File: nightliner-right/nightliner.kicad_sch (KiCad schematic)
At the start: 90 parts, among them J1 TYPE-C-31-M-12, J2 Battery, J3 Serial, J4 Battery, P1 ISP_Prog, SW1 pinky_top, SW10 inner_home, SW11 pinky_bottom, SW12 ring_bottom, SW13 middle_bottom, SW14 index_bottom, SW15 inner_bottom, SW16 outer_top, SW17 outer_home, SW18 near_thumb, SW19 home_thumb, SW2 ring_top, SW20 far_thumb, SW21 ON_OFF, SW22 RESET, SW3 middle_top, SW4 index_top, SW5 inner_top, SW6 pinky_home, SW7 ring_home, SW8 middle_home, SW9 index_home, U1 holyiot-18010, U2 TVS2200DRV, U3 USBLC6-2SC6, U4 BQ24075RGT, U5 XC6220B331MR

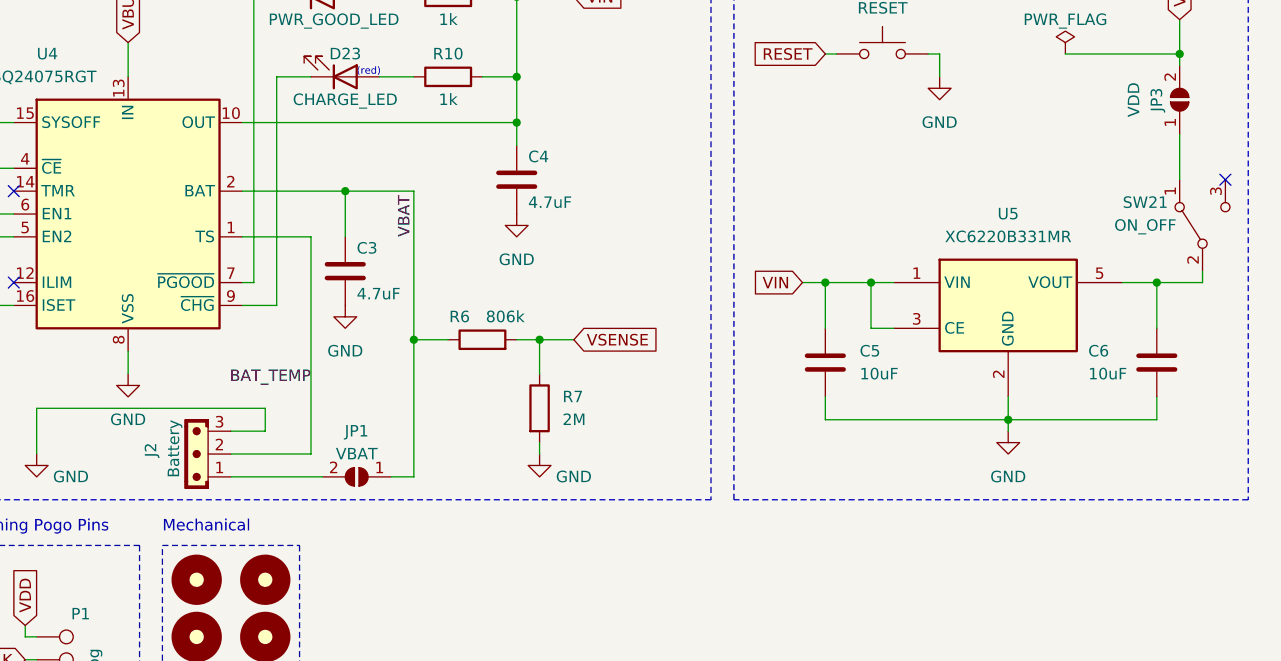
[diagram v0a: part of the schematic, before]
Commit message: fix: final version, create production gerbers
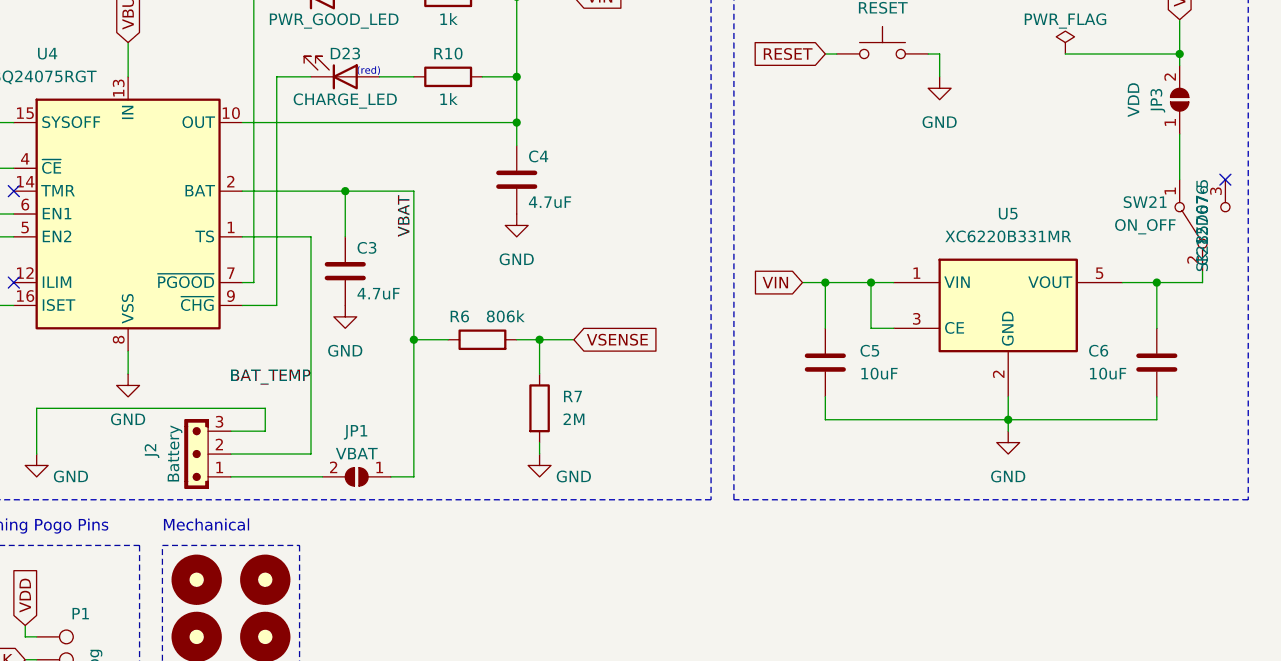
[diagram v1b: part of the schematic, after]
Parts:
- C1: LCSCNumber (none) -> C94121; PartNumber (none) -> CC0805KRX7R9BB102
- C2: LCSCNumber (none) -> C91186; PartNumber (none) -> CC0805KKX7R8BB105
- C3, C4: LCSCNumber (none) -> C354262; PartNumber (none) -> CC0805KKX7R8BB475
- C5, C6, C7: LCSCNumber (none) -> C89831; PartNumber (none) -> CC0805KKX5R8BB106
- D1, D10, D11, D12, D13, D14, D15, D16, D17, D18, D19, D2, D20, D3, D4, D5, D6, D7, D8, D9: value D_Small -> 1N4148WS; LCSCNumber (none) -> C5345963; PartNumber (none) -> 1N4148WS
- D25: LCSCNumber (none) -> C727115; PartNumber (none) -> 1N5819W
- H1: footprint miro_keyboard:StandOff_6mm_M3 -> nightliner:StandOff_6mm_M3
- H2, H3, H4, H5, H6, H7: value MountingHole_M3 -> Standoff_6mm_M3; footprint miro_keyboard:StandOff_6mm_M3 -> nightliner:StandOff_6mm_M3
- J1: symbol Connector:USB_C_Receptacle_USB2.0 -> nightliner:USB_C_Receptacle_USB2.0
- J2: LCSCNumber (none) -> C163036; PartNumber (none) -> S3B-XH-A-1(LF)(SN)
- J3: footprint miro_keyboard:MagConn_6pin_right -> nightliner:MagConn_6pin_right
- P1: footprint miro_keyboard:ISP_Programming_Pads -> nightliner:ISP_Programming_Pads
- R1, R2: LCSCNumber (none) -> C144553; PartNumber (none) -> AC0805FR-075K1L
- R10, R11, R8, R9: LCSCNumber (none) -> C95781; PartNumber (none) -> RC0805FR-071KL
- R3: LCSCNumber (none) -> C107700; PartNumber (none) -> RC0805FR-071ML
- R4: LCSCNumber (none) -> C140868; PartNumber (none) -> AC0805FR-0710KL
- R6: LCSCNumber (none) -> C273852; PartNumber (none) -> RC0805FR-07806KL
- R7: LCSCNumber (none) -> C114532; PartNumber (none) -> RC0805FR-072ML
- SW1, SW10, SW11, SW12, SW13, SW14, SW15, SW16, SW17, SW18, SW19, SW2, SW20, SW3, SW4, SW5, SW6, SW7, SW8, SW9: footprint miro_keyboard:Kailh_Choc_CPG135001D02_Hotswap -> nightliner:Kailh_Choc_CPG135001D02_Hotswap
- SW21: footprint miro_keyboard:SW_ROCPU_SK-12D07-5_SPDT_Angled -> nightliner:SW_ROCPU_SK-12D07-5_SPDT_Angled; LCSCNumber (none) -> C2857676; PartNumber (none) -> SK-12D07-5
- SW22: footprint miro_keyboard:SW_Push_1P1T_NO_CK_KSC4xxJ -> nightliner:SW_Push_1P1T_NO_CK_KSC4xxJ
- U1: footprint miro_keyboard:HOLYIOT-18010-UndersidePins-SMD -> nightliner:HOLYIOT-18010-UndersidePins-SMD
- U2: LCSCNumber (none) -> C523793; PartNumber (none) -> TVS2200DRVR
- U3: LCSCNumber (none) -> C7519; PartNumber (none) -> USBLC6-2SC6
- U4: footprint miro_keyboard:VQFN-16-1EP_3x3mm_P0.5mm_EP1.6x1.6mm_ThermalVias -> nightliner:VQFN-16-1EP_3x3mm_P0.5mm_EP1.6x1.6mm_ThermalVias; LCSCNumber (none) -> C15464; PartNumber (none) -> BQ24075RGTR
- U5: LCSCNumber (none) -> C86534; PartNumber (none) -> XC6220B331MR-G
